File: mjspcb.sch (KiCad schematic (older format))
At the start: 153 parts, among them J1 FTDI, J10 Analog, J12 SWD, J13 Conn_Coaxial, J14 Lithium Ion, J15 Temp/Hum, J16 BPW34, J17 USB_C_connector, J18 I2C 3V_perm, J19 I2C 5V_SW, J2 Conn_01x16_Female, J20 Multi, J3 Conn_01x02_Male, J4 Oled, J5 Conn_01x02_Male, J6 Solar, J7 Particulate matter, J8 Prototype power, J9 Prototype GND, Q1 DMP2035U-7, Q2 DMP2035U-7, SW1 SW_Push, SW2 SW_Push, SW3 SW_Push, U1 USBLC-2SC6, U2 LoRa_1262_G-NiceRF, U3 GPS, U4 PrototypeGrid, U5 STM32L072RZTx-meetjestad, U6 MCP73831, U7 MCP9808_MSOP, U8 SST26VF032B, Y1 32kHz

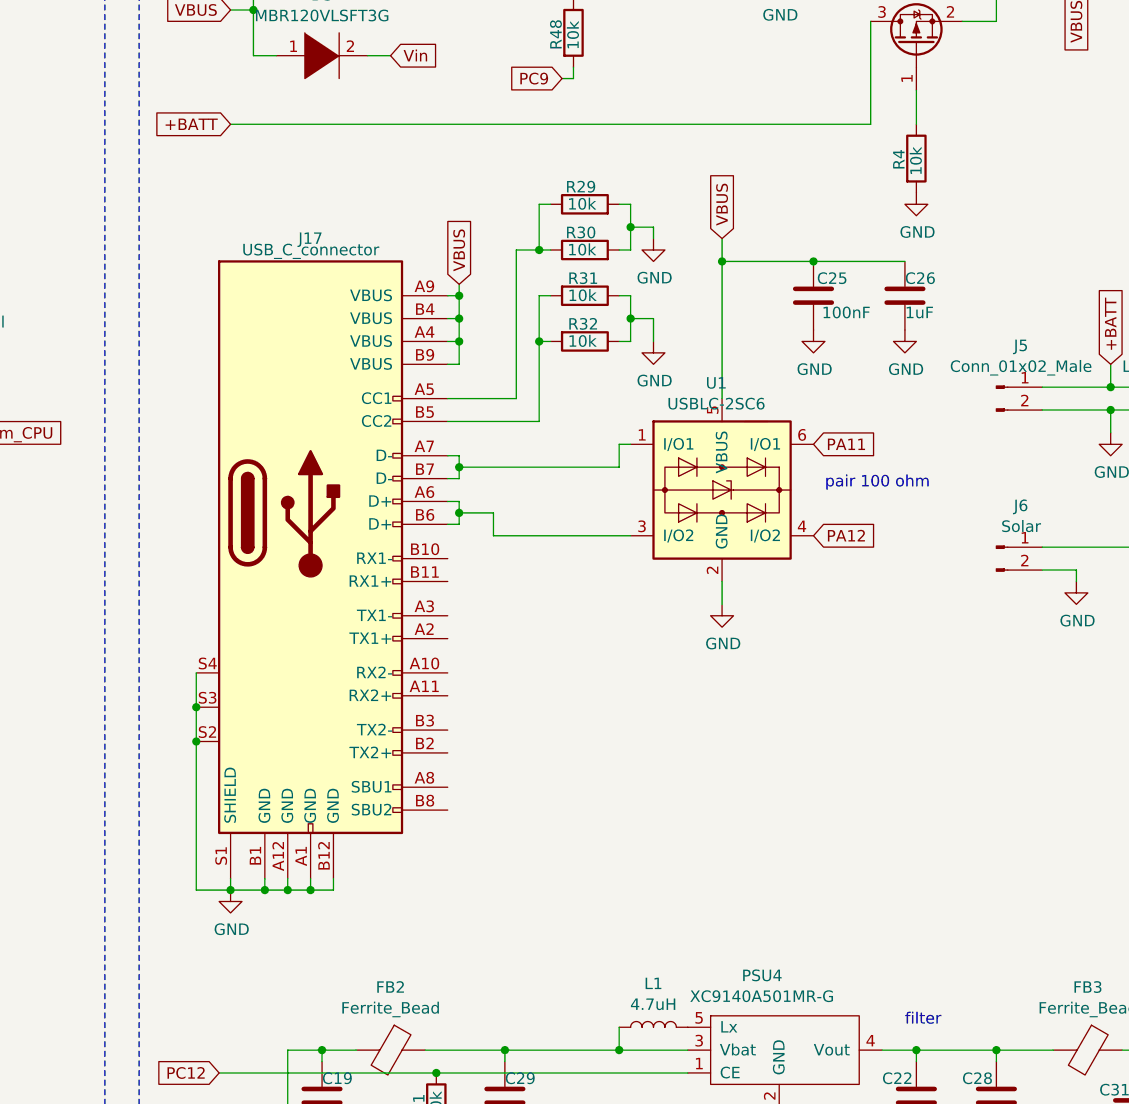
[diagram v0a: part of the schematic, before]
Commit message: Update to MJS2020-PROTO4
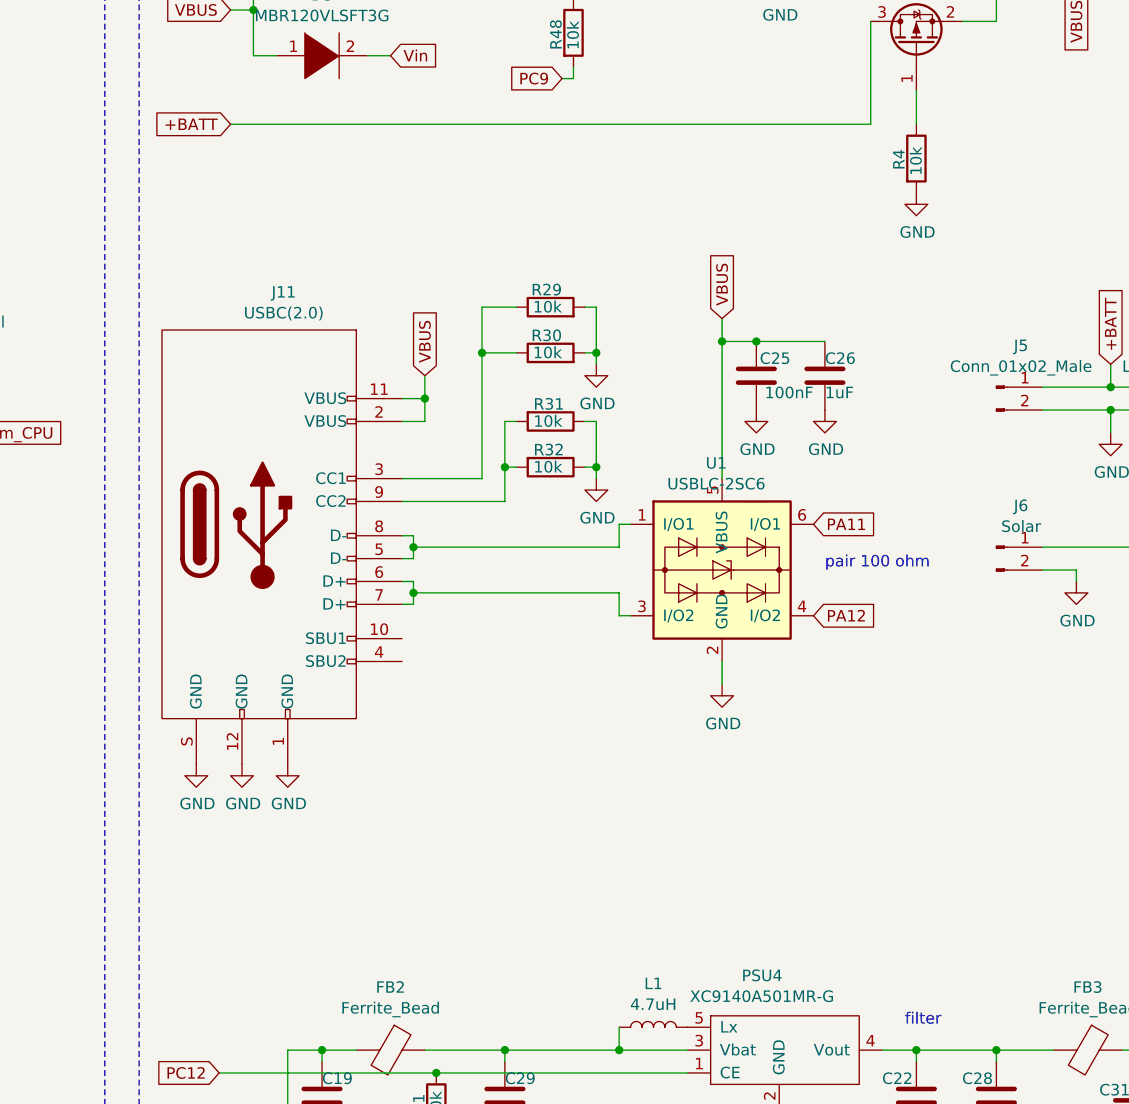
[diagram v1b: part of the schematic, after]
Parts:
- removed J17: USB_C_connector, meetjestad:USB-C_new, symbol meetjestad:USB_C_connector
- added J11: USBC(2.0), meetjestad:DX07S016JA3R1500, symbol mjspcb-rescue:USBC(2.0)-meetjestad
- H1, H2, H3: footprint MountingHole:MountingHole_3.2mm_M3 -> meetjestad:MountingHole_3.2mm_M3
- J15: footprint meetjestad:SI7021 -> meetjestad2:SI7021
- J16, J3: footprint Connector_PinHeader_2.54mm:PinHeader_1x02_P2.54mm_Vertical -> meetjestad:PinHeader_Male_1X2
- J2: footprint Connector_PinSocket_2.54mm:PinSocket_1x16_P2.54mm_Vertical -> meetjestad:PinHeader_Female_1X16
- J5: footprint meetjestad:Battery__holder -> meetjestad2:Battery__holder
- J8, J9: footprint Connector_PinSocket_2.54mm:PinSocket_1x06_P2.54mm_Vertical -> meetjestad:PinHeader_Female_1X6
- SW1, SW2: footprint Button_Switch_THT:SW_PUSH_6mm -> meetjestad:SW_Push_6mm
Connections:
- net GND: now also J11.1 (GND), J11.12 (GND), J11.S (GND)
- net VBUS: now also J11.11 (VBUS), J11.2 (VBUS)
- net at R29.1, R30.1: now also J11.3 (CC1)
- net at R31.2, R32.2: now also J11.9 (CC2)
- net at U1.3 (I/O2): now also J11.6 (D+), J11.7 (D+)
- net at U1.1 (I/O1): now also J11.5 (D-), J11.8 (D-)
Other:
- moved on the sheet: C25, C26, R29, R30, R31, R32, U1
